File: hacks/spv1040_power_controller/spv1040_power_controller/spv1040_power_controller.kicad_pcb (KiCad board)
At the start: 2 copper layers, 37.8 x 22.1 mm, 21 parts, among them SW1 SWITCH_INV, U1 SPV1040

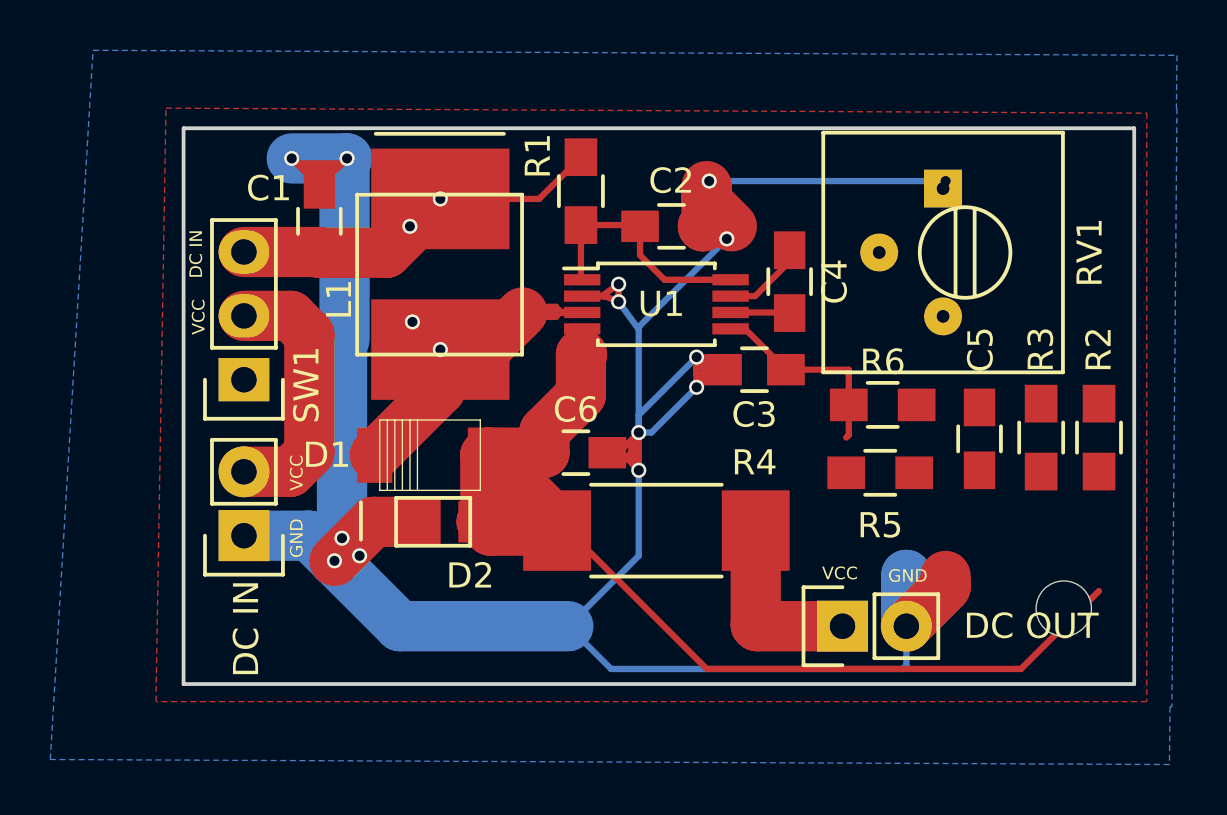
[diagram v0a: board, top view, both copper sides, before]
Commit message: ordered spv1040 pcb
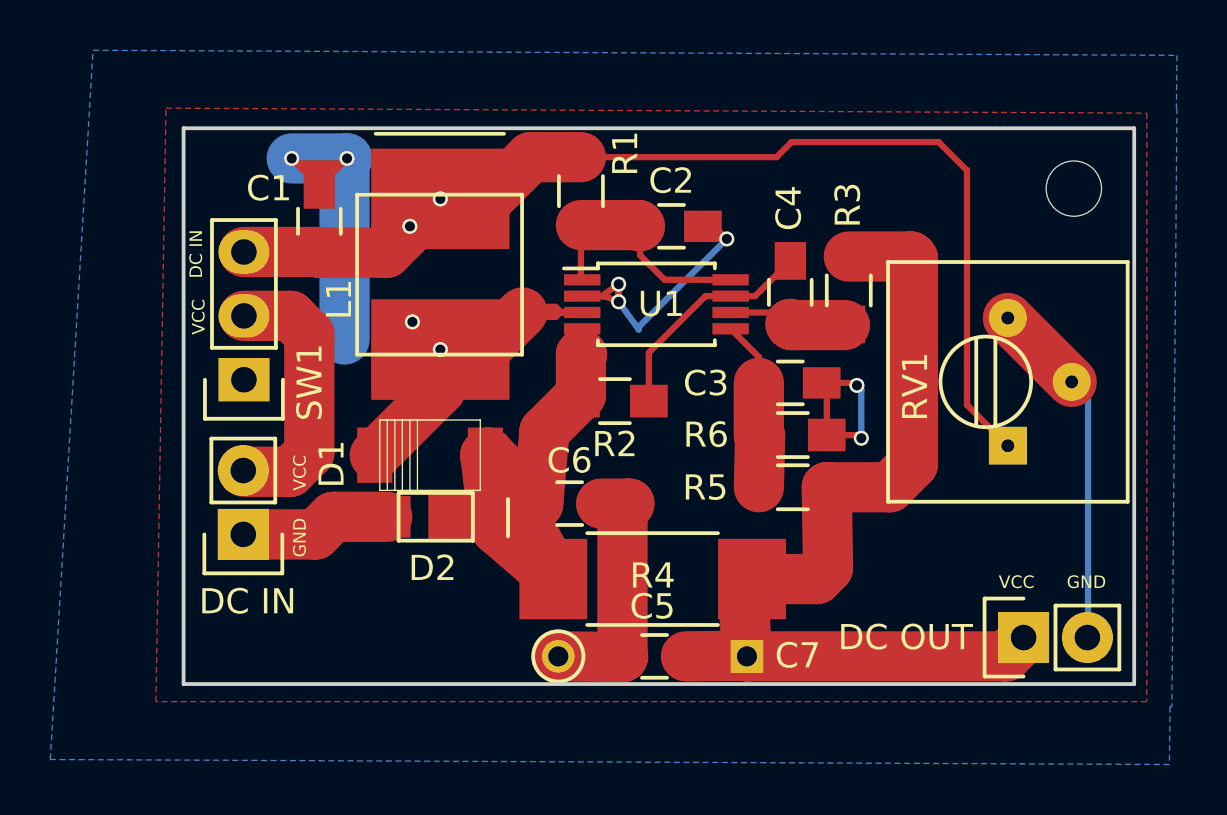
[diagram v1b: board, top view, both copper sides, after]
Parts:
- added C7: 4700uF, 4700uF_16mm:C_Radial_D16_L25_P7.5, F.Cu at (182.4, 126.9)
- moved R2 19.3 mm to (177.2, 116.8), turned to 0 degrees
- moved REF** 16.7 mm to (195.4, 108.3)
- moved C5 15.6 mm to (178.7, 126.9), turned to 180 degrees
- moved RV1 10.5 mm to (192.8, 118.5), turned to 90 degrees
- moved R3 9.63 mm to (186.4, 112.3), turned to 270 degrees
- moved DC OUT 7.21 mm to (193.4, 126.2)
- moved R6 3.77 mm to (184.2, 118.1)
- moved D2 3.54 mm to (168.6, 120.4), turned to 0 degrees
- moved R5 3.52 mm to (184.2, 120.2)
- moved C6 2.04 mm to (175.3, 120.8)
- moved R4 1.93 mm to (178.7, 123.8)
- moved C3 1.52 mm to (184.1, 116.0), turned to 0 degrees
- moved C4 0.43 mm to (184.1, 112.4)
- moved DC IN 0.06 mm to (162.4, 122.0)
- turned R1 to 270 degrees
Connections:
- D2 pad 1: Net-(C6-Pad1) -> GND
- D2 pad 2: GND -> Net-(C6-Pad1)
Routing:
- net Net-(C1-Pad1): track 83.1 -> 48.1 mm, vias 12 -> 2
- net Net-(C5-Pad1): track 7.22 -> 38.0 mm
- net Net-(C6-Pad1): track 44.0 -> 23.6 mm
- net Net-(C4-Pad1): track 3.37 -> 9.06 mm
- net GND: track 72.8 -> 68.3 mm, vias 4 -> 7
- net Net-(C4-Pad2): track 2.36 -> 4.76 mm
- net Net-(C2-Pad1): track 7.64 -> 9.93 mm
- net Net-(C3-Pad1): track 8.11 -> 7.36 mm
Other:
- rule pad_to_mask_clearance: 0.2 -> 0.0508
- board text added: "Solar cell power controller using SPV1040 by @mik4el4ndersson 2016 V01. DC IN max 3V 1A DC OUT max 5V"
- board text removed: "Solar cell power controller using SPV1040 by @mik4el4ndersson 2016 V01. DC IN max 3V 1A DC OUT max 5V 100mA"
